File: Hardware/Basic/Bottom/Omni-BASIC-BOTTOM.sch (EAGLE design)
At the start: 32 parts, among them U1 AD5242-SO16

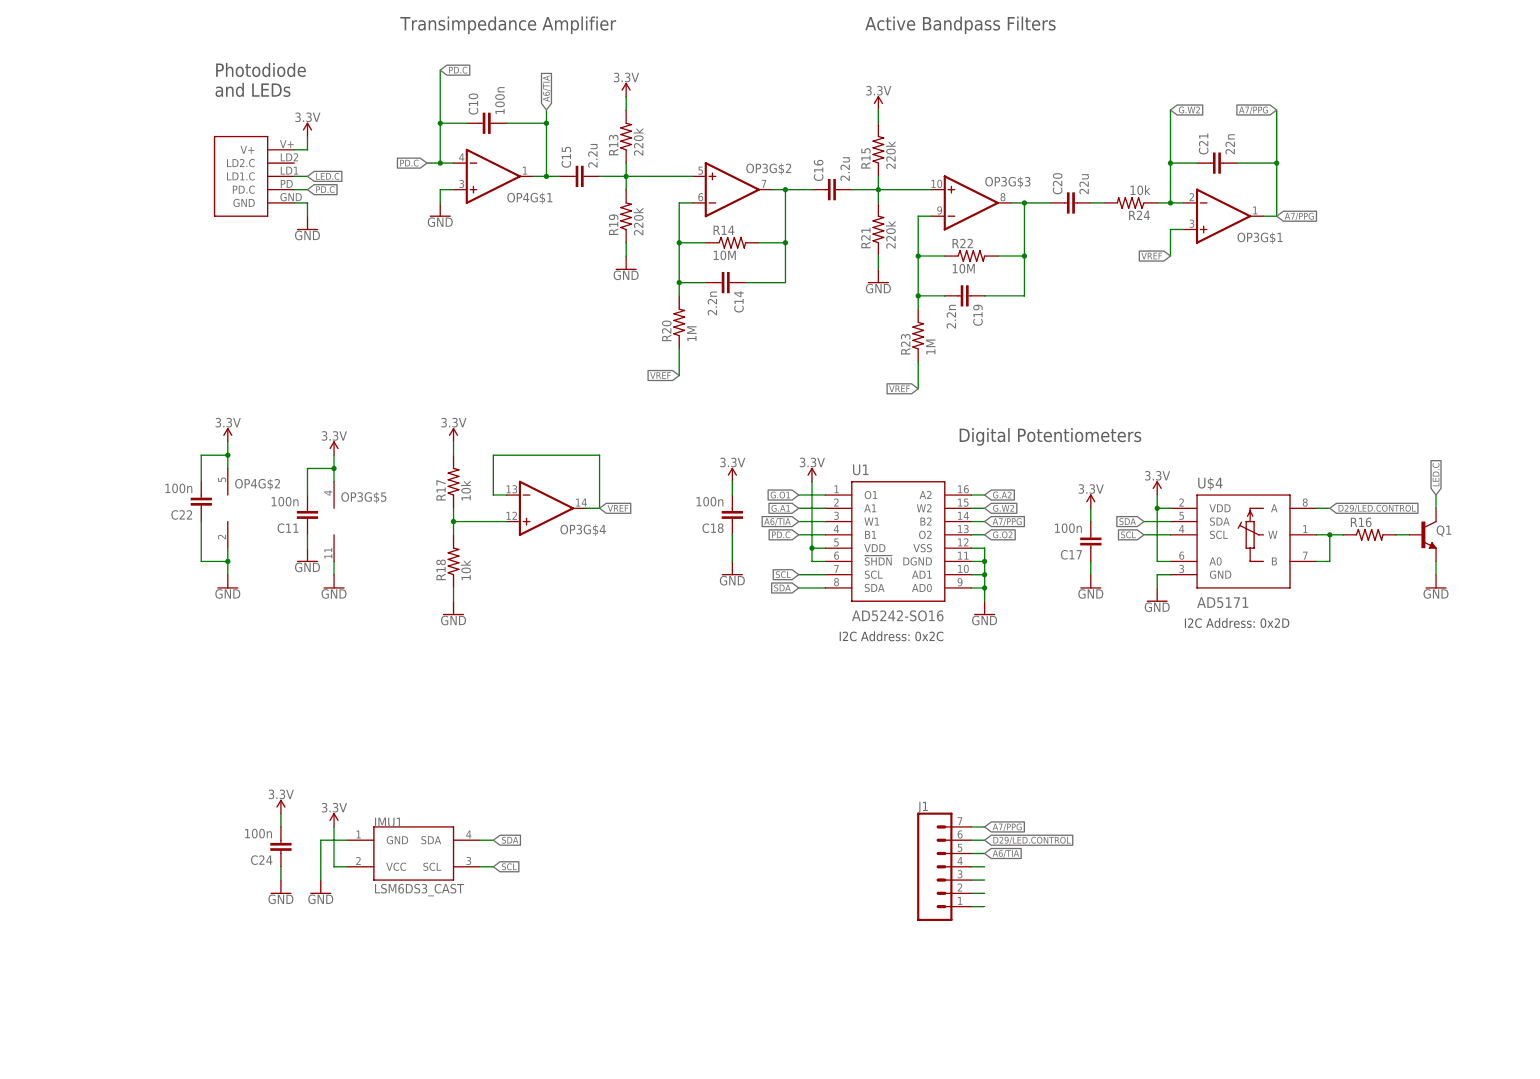
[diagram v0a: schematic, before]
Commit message: Latest Update
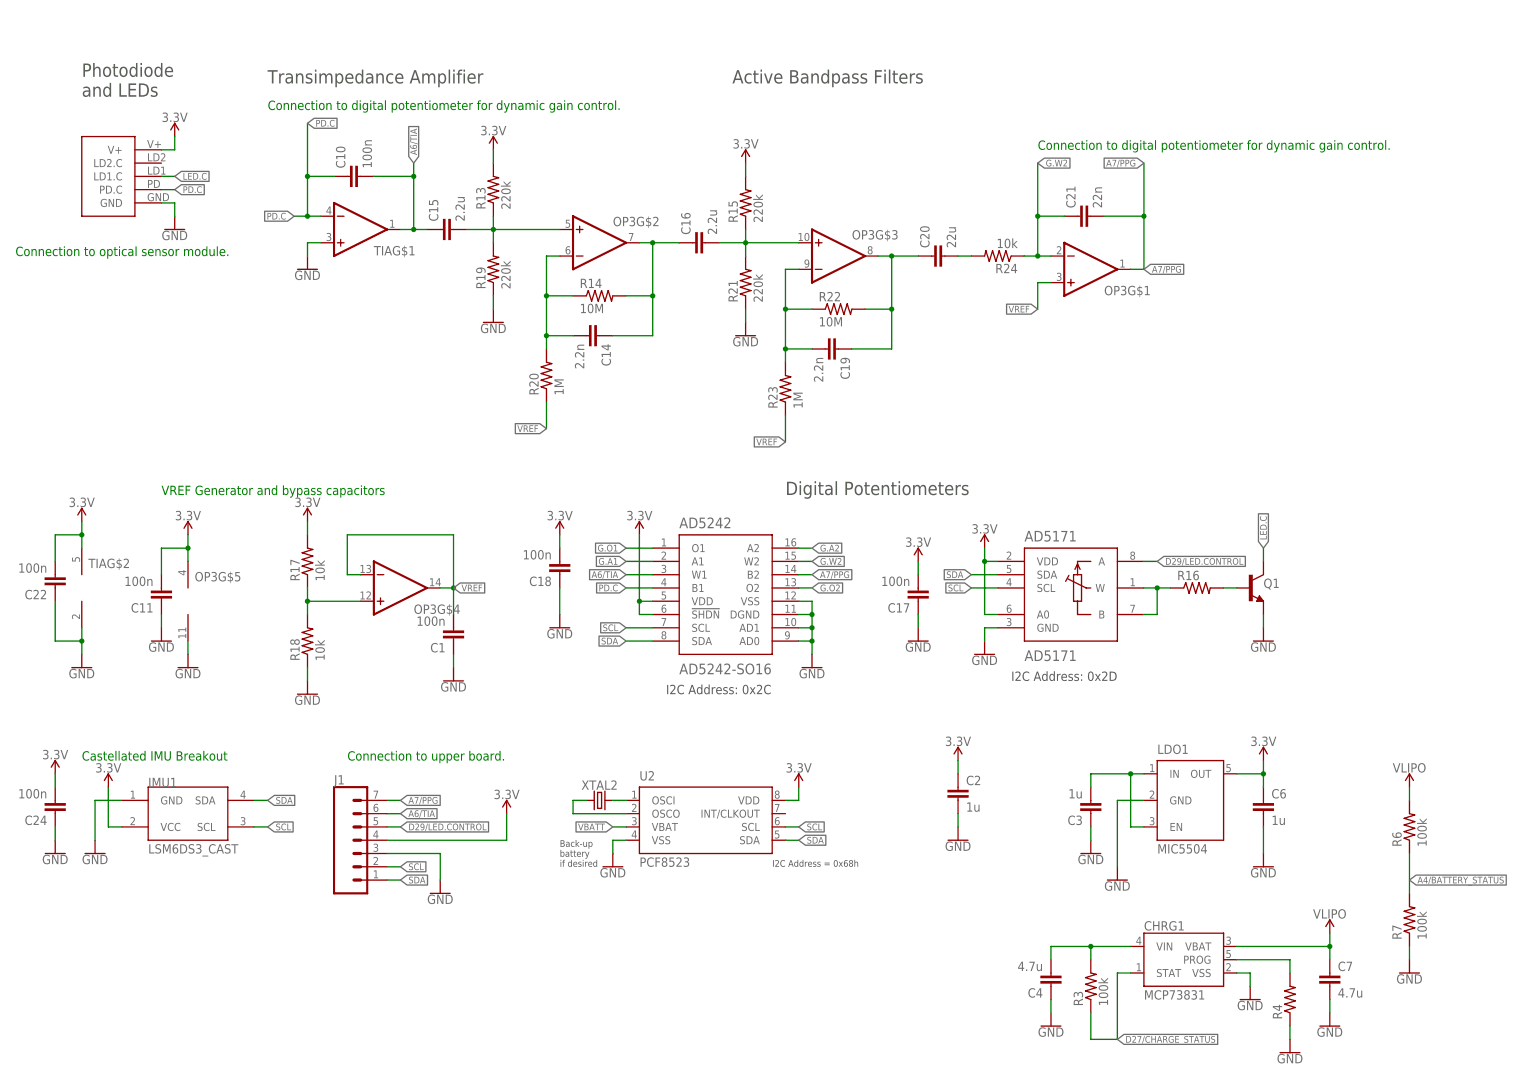
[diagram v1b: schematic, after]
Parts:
- removed OP4: (no value), LinnesLab-AnalogIC:OP-SINGLEOT
- removed U$4: AD5171, LinnesLab-DigitalIC:AD5171
- removed U1: AD5242-SO16, LinnesLab-DigitalIC:AD5242-SO16
- added AD5171: AD5171, LinnesLab-DigitalIC:AD5171
- added AD5242: AD5242-SO16, LinnesLab-DigitalIC:AD5242-SO16
- added C1: 100n, LinnesLab-Passives:CAPACITOR0603
- added C2, C3, C6: 1u, LinnesLab-Passives:CAPACITOR0603
- added C4, C7: 4.7u, LinnesLab-Passives:CAPACITOR0603
- added CHRG1: MCP73831, LinnesLab-Power:MCP73831
- added LDO1: MIC5504, LinnesLab-Power:MIC5504
- added R3, R6, R7: 100k, LinnesLab-Passives:RESISTOR0603
- added R4: (no value), LinnesLab-Passives:RESISTOR0603
- added TIA: (no value), LinnesLab-AnalogIC:OP-SINGLEOT
- added U2: PCF8523, LinnesLab-Clocks:PCF8523
- added XTAL2: 32.7680kHz, LinnesLab-Clocks:CRYSTALECS-.327-12.5-12-C-TR
- J1: device LinnesLab-Connectors:CONN_07 -> LinnesLab-Connectors:CONN_07-1.27MM
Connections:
- removed net N$7: J1.1
- new net A4/BATTERY_STATUS: R6.1, R7.2
- new net D27/CHARGE_STATUS: CHRG1.STAT, R3.1
- new net N$3: U2.OSCO, XTAL2.1
- new net VBATT: U2.VBAT
- new net VIN1: C4.2, CHRG1.VIN, R3.2
- new net VLIPO: C7.1, CHRG1.VBAT, R6.2
- net 3.3V: now also AD5171.A0, AD5171.VDD, AD5242.!SHDN, AD5242.VDD, C2.1, C6.1, J1.4, LDO1.OUT, TIAG$2.V+, U2.VDD; no longer OP4G$2.V+, U$4.A0, U$4.VDD, U1.!SHDN, U1.VDD
- net A6/TIA: now also AD5242.W1, J1.6, TIAG$1.OUT; no longer J1.5, OP4G$1.OUT, U1.W1
- net A7/PPG: now also AD5242.B2; no longer U1.B2
- net D29/LED.CONTROL: now also AD5171.A, J1.5; no longer J1.6, U$4.A
- net G.A1: now also AD5242.A1; no longer U1.A1
- net G.A2: now also AD5242.A2; no longer U1.A2
- net G.O1: now also AD5242.O1; no longer U1.O1
- net G.O2: now also AD5242.O2; no longer U1.O2
- net G.W2: now also AD5242.W2; no longer U1.W2
- net GND: now also AD5171.GND, AD5242.AD0, AD5242.AD1, AD5242.DGND, AD5242.VSS, C1.1, C2.2, C3.1, C4.1, C6.2, C7.2, CHRG1.VSS, J1.3, LDO1.GND, R4.1, R7.1, TIAG$1.+IN, TIAG$2.V-, U2.VSS; no longer OP4G$1.+IN, OP4G$2.V-, U$4.GND, U1.AD0, U1.AD1, U1.DGND, U1.VSS
- net N$4: now also U2.OSCI, XTAL2.2; no longer J1.4
- net N$5: now also CHRG1.PROG, R4.2; no longer J1.3
- net N$6: now also C3.2, LDO1.EN, LDO1.IN; no longer J1.2
- net N$9: now also AD5171.B, AD5171.W; no longer U$4.B, U$4.W
- net PD.C: now also AD5242.B1, TIAG$1.-IN; no longer OP4G$1.-IN, U1.B1
- net SCL: now also AD5171.SCL, AD5242.SCL, J1.2, U2.SCL; no longer U$4.SCL, U1.SCL
- net SDA: now also AD5171.SDA, AD5242.SDA, J1.1, U2.SDA; no longer U$4.SDA, U1.SDA
- net VREF: now also C1.2
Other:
- note added: "Back-up battery if desired"
- note added: "Castellated IMU Breakout"
- note added: "Connection to digital potentiometer for dynamic gain control."
- note added: "Connection to optical sensor module."
- note added: "Connection to upper board."
- note added: "I2C Address = 0x68h"
- note added: "VREF Generator and bypass capacitors"
- moved on the sheet: C10, C11, C14, C15, C16, C17, C18, C19, C20, C21, C22, C24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
